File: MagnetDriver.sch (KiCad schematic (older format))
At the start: 59 parts, among them J1 MAGNET1, J2 MAGNET2, J3 INPUT_JACK, J4 PWR_IN, Q1 2N3904, Q2 TIP122, Q3 TIP32A, Q4 2N3904, Q5 TIP122, Q6 TIP32A, U1 LM324, U2 TEENSY_3.6_MINIMAL, U3 LM7805_TO220

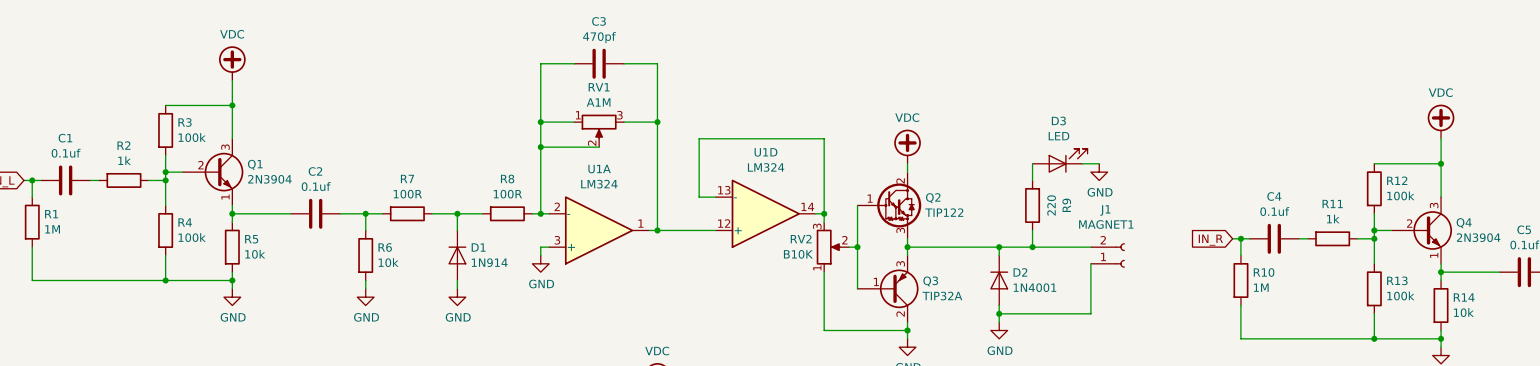
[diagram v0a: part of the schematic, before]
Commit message: placed components
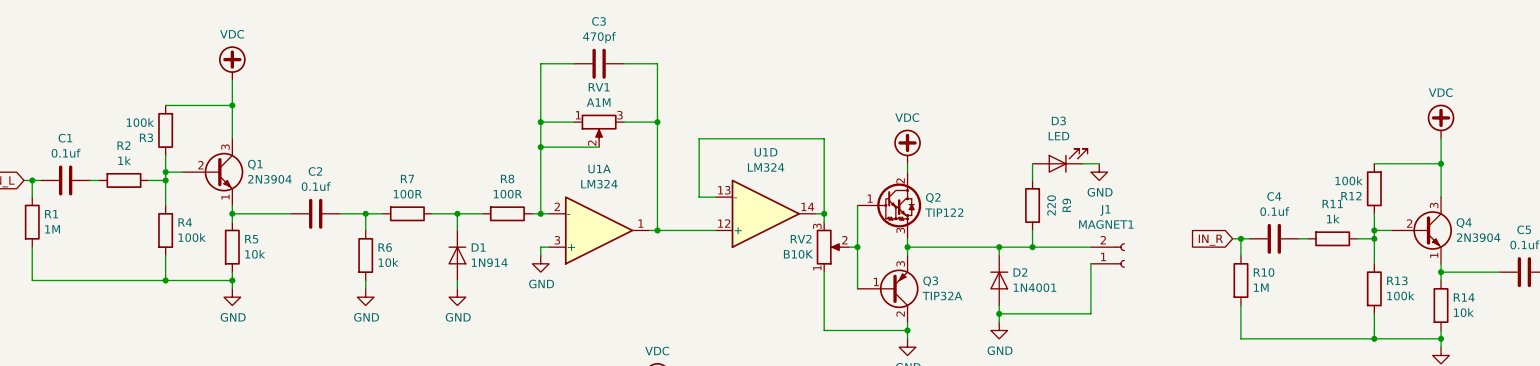
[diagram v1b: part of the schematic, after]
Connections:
- net VDC: now also R12.2, R3.2; no longer R12.1, R3.1
- net at Q1.2 (B), R2.1, R4.1: now also R3.1; no longer R3.2
- net at Q4.2 (B), R11.1, R13.1: now also R12.1; no longer R12.2
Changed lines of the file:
@@
 F 3 "~" H 2050 1800 50  0001 C CNN
 	1    2050 1800
-	1    0    0    -1
+	-1   0    0    1
 $EndComp
 $Comp
@@
 F 3 "~" H 9300 2150 50  0001 C CNN
 	1    9300 2150
-	1    0    0    -1
-$EndComp
-$Comp
+	-1   0    0    1
+$EndComp
+$Comp

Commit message: backup before layout changes
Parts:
- removed U3: LM7805_TO220, Package_TO_SOT_THT:TO-220-3_Horizontal_TabDown, symbol Regulator_Linear:LM7805_TO220
- added D9: DNP, LED_THT:LED_D5.0mm, symbol Device:LED
- added Q7: DNP, Package_TO_SOT_THT:TO-92_Inline, symbol Transistor_BJT:2N3904
- added R20, R21, R22: DNP, HammerheadAudio:R_THT_P7.62, symbol Device:R
- added SW1: DNP, HammerheadAudio:Tayda_Slide_SPDT, symbol Switch:SW_SPDT
- added U3: R-78E5.0-0.5, Converter_DCDC:Converter_DCDC_RECOM_R-78E-0.5_THT, symbol Regulator_Switching:R-78E5.0-0.5
- C1, C11, C2, C4, C5: CSV (none) -> C1620173; LCSC (none) -> C1620173
- C3, C6: CSV (none) -> C1620141; LCSC (none) -> C1620141
- C7, C8: value 10uf -> DNP
- C9: CSV (none) -> C2761740; LCSC (none) -> C2761740
- D1, D4: CSV (none) -> C258180; LCSC (none) -> C258180
- D2, D5, D7: CSV (none) -> C2456; LCSC (none) -> C2456
- D3, D6, D8: CSV (none) -> C2895493; LCSC (none) -> C2895493
- J1, J2, J4: CSV (none) -> C430324; LCSC (none) -> C430324
- J3: CSV (none) -> C16684; LCSC (none) -> C16684
- Q1, Q4: CSV (none) -> C2874602; LCSC (none) -> C2874602
- Q2, Q5: CSV (none) -> C16283; LCSC (none) -> C16283
- Q3, Q6: CSV (none) -> C2927632; LCSC (none) -> C2927632
- R11, R2: CSV (none) -> C2894541; LCSC (none) -> C2894541
- R12, R13, R3, R4: CSV (none) -> C714036; LCSC (none) -> C714036
- R14, R15, R5, R6: CSV (none) -> C172967; LCSC (none) -> C172967
- R16, R17, R7, R8: CSV (none) -> C57438; LCSC (none) -> C57438
- R18, R19, R9: value 220 -> 1k; CSV (none) -> C2894541; LCSC (none) -> C2894541
- RV1, RV2, RV3, RV4: CSV (none) -> C5205027; LCSC (none) -> C5205027
- U1: CSV (none) -> C132508; LCSC (none) -> C132508
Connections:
- net +5V: now also SW1.2 (B), U3.3 (OUT); no longer U2.48 (Vin)
- net GND: now also D9.1 (K), Q7.1 (E), R22.1, U3.2 (GND)
- net VDC: now also U3.1 (IN)
- net at U2.44 (22_A8_PWM_Touch): now also Q7.3 (C)
- net at U2.45 (23_A9_PWM_Touch): now also R20.2
- new net: SW1.3 (C), U2.48 (Vin)
- new net: R21.2, SW1.1 (A)
- new net: D9.2 (A), R20.1
- new net: Q7.2 (B), R21.1, R22.2
- no-connect marks 43 -> 41
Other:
- moved on the sheet: C10, C7, C8, C9, D7, D8, H1, H2, H3, H4, J3, J4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
